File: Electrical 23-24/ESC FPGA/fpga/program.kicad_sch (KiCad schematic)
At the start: 8 parts, among them SW2 SW_Push, U1 XC6SLX4-TQG144

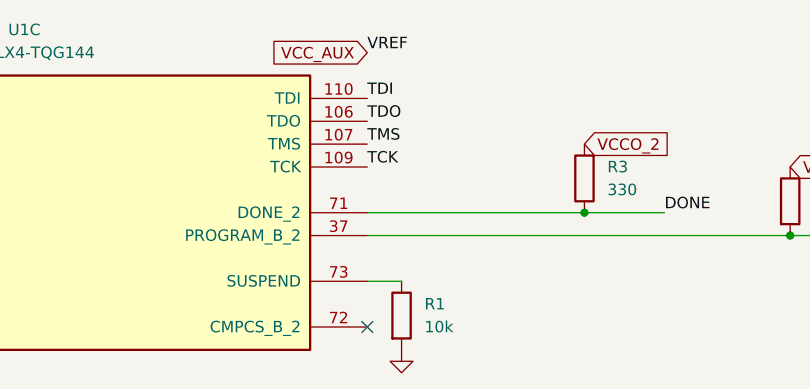
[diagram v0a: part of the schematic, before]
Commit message: Add programmer
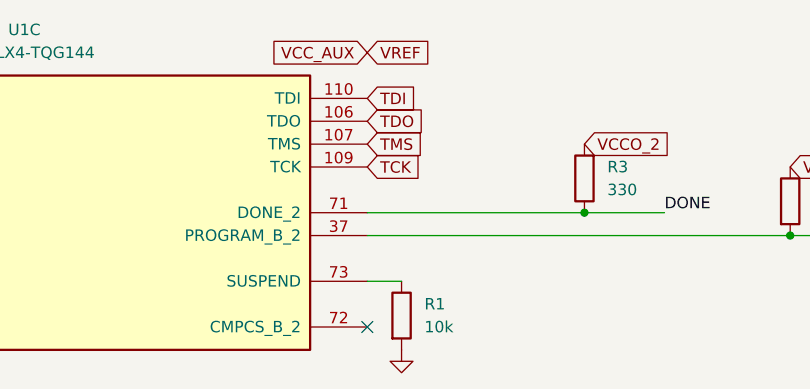
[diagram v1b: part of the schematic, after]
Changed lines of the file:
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@@
     (effects (font (size 2.54 2.54)) (justify left bottom))
   )
-  (label "TCK" (at 179.07 85.09 0) (fields_autoplaced)
-    (effects (font (size 1.27 1.27)) (justify left bottom))
-  )
-  (label "TDO" (at 179.07 80.01 0) (fields_autoplaced)
-    (effects (font (size 1.27 1.27)) (justify left bottom))
-  )
   (label "DONE" (at 212.09 90.17 0) (fields_autoplaced)
-    (effects (font (size 1.27 1.27)) (justify left bottom))
-  )
-  (label "TMS" (at 179.07 82.55 0) (fields_autoplaced)
-    (effects (font (size 1.27 1.27)) (justify left bottom))
-  )
-  (label "TDI" (at 179.07 77.47 0) (fields_autoplaced)
-    (effects (font (size 1.27 1.27)) (justify left bottom))
-  )
-  (label "VREF" (at 179.07 72.39 0) (fields_autoplaced)
     (effects (font (size 1.27 1.27)) (justify left bottom))
   )
@@
     )
   )
+  (global_label "TCK" (shape input) (at 179.07 85.09 0) (fields_autoplaced)
+    (effects (font (size 1.27 1.27)) (justify left))
+    (property "Intersheetrefs" "${INTERSHEET_REFS}" (at 185.5628 85.09 0)
+      (effects (font (size 1.27 1.27)) (justify left) hide)
+    )
+  )
+  (global_label "TMS" (shape input) (at 179.07 82.55 0) (fields_autoplaced)
+    (effects (font (size 1.27 1.27)) (justify left))
+    (property "Intersheetrefs" "${INTERSHEET_REFS}" (at 185.6837 82.55 0)
+      (effects (font (size 1.27 1.27)) (justify left) hide)
+    )
+  )
+  (global_label "TDI" (shape input) (at 179.07 77.47 0) (fields_autoplaced)
+    (effects (font (size 1.27 1.27)) (justify left))
+    (property "Intersheetrefs" "${INTERSHEET_REFS}" (at 184.8976 77.47 0)
+      (effects (font (size 1.27 1.27)) (justify left) hide)
+    )
+  )
+  (global_label "VREF" (shape input) (at 179.07 72.39 0) (fields_autoplaced)
+    (effects (font (size 1.27 1.27)) (justify left))
+    (property "Intersheetrefs" "${INTERSHEET_REFS}" (at 186.6514 72.39 0)
+      (effects (font (size 1.27 1.27)) (justify left) hide)
+    )
+  )
   (global_label "VCC_AUX" (shape input) (at 179.07 72.39 180) (fields_autoplaced)
     (effects (font (size 1.27 1.27)) (justify right))
@@
     )
   )
+  (global_label "TDO" (shape input) (at 179.07 80.01 0) (fields_autoplaced)
+    (effects (font (size 1.27 1.27)) (justify left))
+    (property "Intersheetrefs" "${INTERSHEET_REFS}" (at 185.6233 80.01 0)
+      (effects (font (size 1.27 1.27)) (justify left) hide)
+    )
+  )
